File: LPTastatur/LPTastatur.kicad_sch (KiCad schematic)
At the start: 23 parts, among them J1 Conn_01x04, Q1 BC556, SW1 SW_Push_Dual, SW2 SW_Push_Dual, SW3 SW_Push_Dual, U1 L7805, U2 NE555P

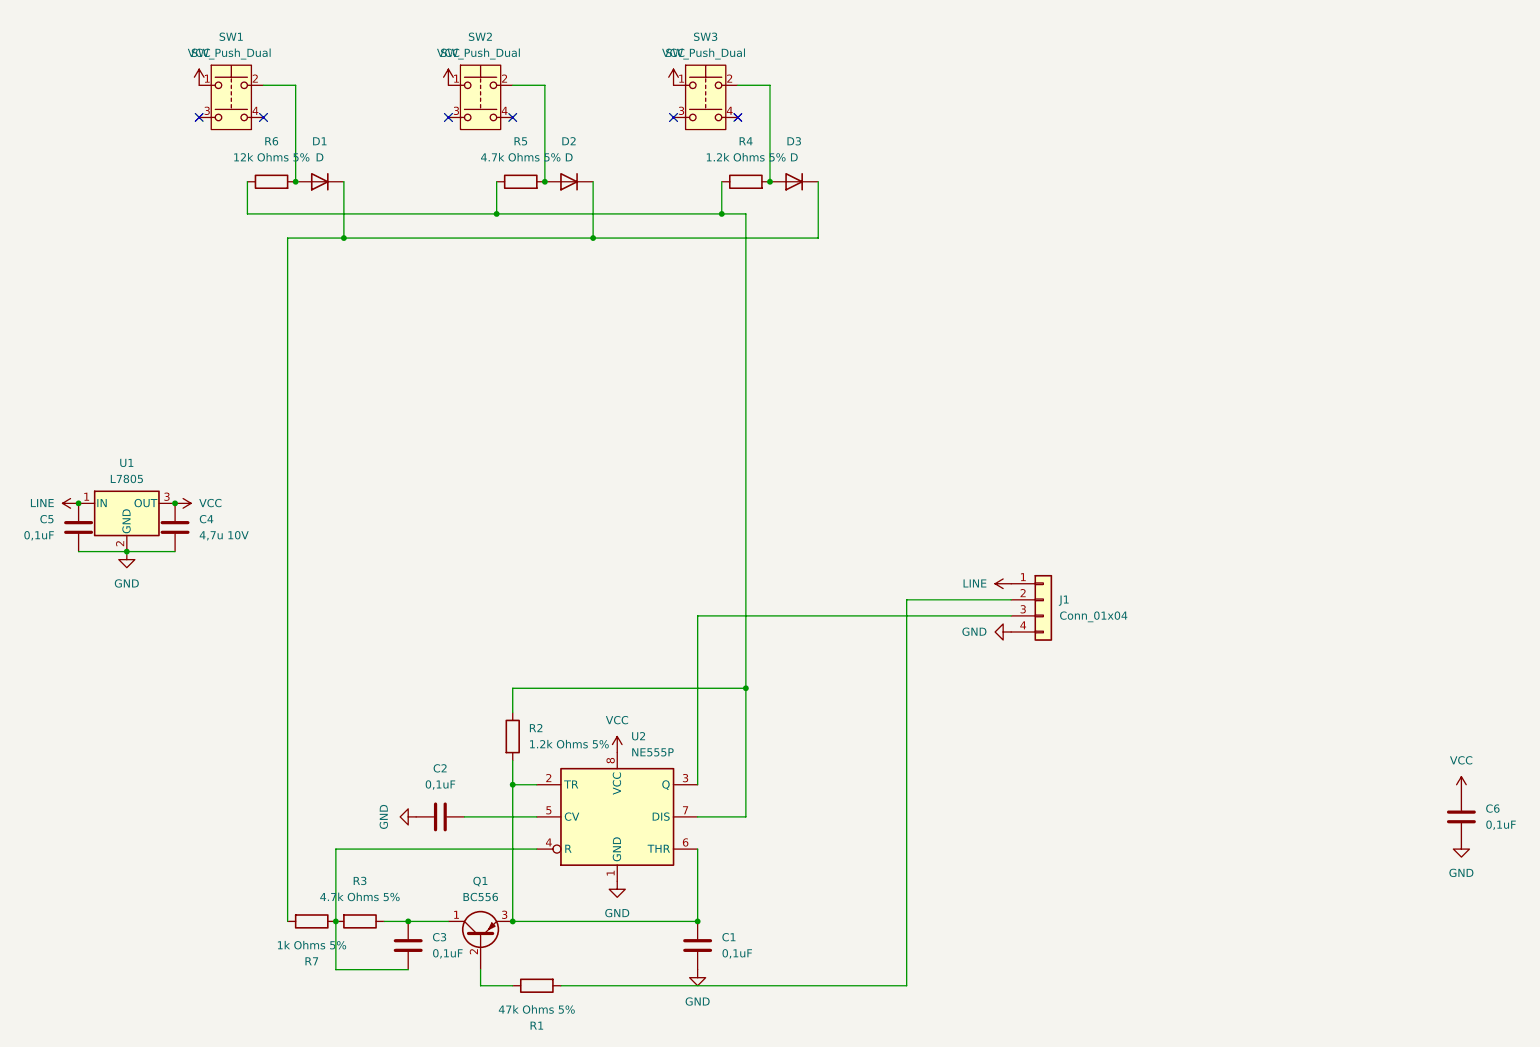
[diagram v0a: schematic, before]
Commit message: din a5
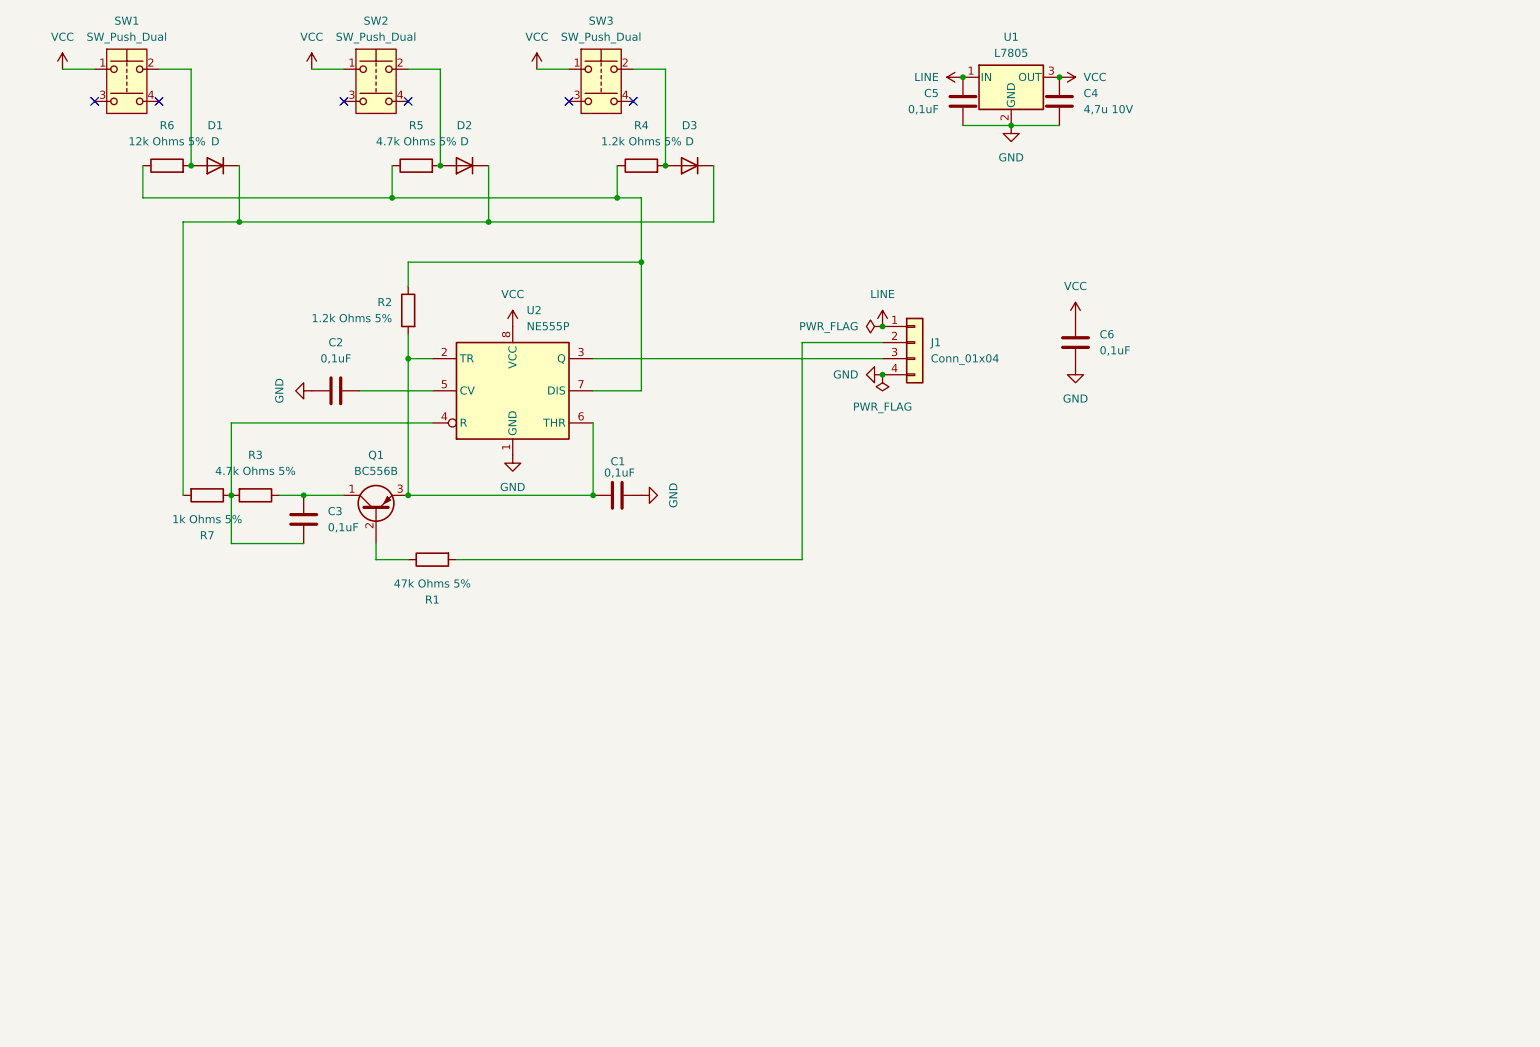
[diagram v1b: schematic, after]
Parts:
- Q1: value BC556 -> BC556B
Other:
- moved on the sheet: C1, C2, C3, C4, C5, C6, D1, D2, D3, J1, Q1, R1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

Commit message: sieht besser aus im 3d render
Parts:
- J1: footprint Connector_PinSocket_2.54mm:PinSocket_1x04_P2.54mm_Vertical -> Connector_PinHeader_2.54mm:PinHeader_1x04_P2.54mm_Horizontal
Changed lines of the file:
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@@
 			)
 		)
-		(property "Footprint" "Connector_PinSocket_2.54mm:PinSocket_1x04_P2.54mm_Vertical"
+		(property "Footprint" "Connector_PinHeader_2.54mm:PinHeader_1x04_P2.54mm_Horizontal"
 			(at 151.13 66.04 0)
 			(effects
